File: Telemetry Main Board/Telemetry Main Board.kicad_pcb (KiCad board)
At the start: 2 copper layers, 107 x 144.2 mm, 26 parts, among them J1 8 pin ATM connector, J3 12 pin ATM connector, J4 SD to SPI (Molex nanofit), U1 LM7805_TO220, U2 LM7809_TO220, U3 NUCLEO-F446RE, U4 ISO1050DUB, U6 MCP6004, U8 ISO1050DUB

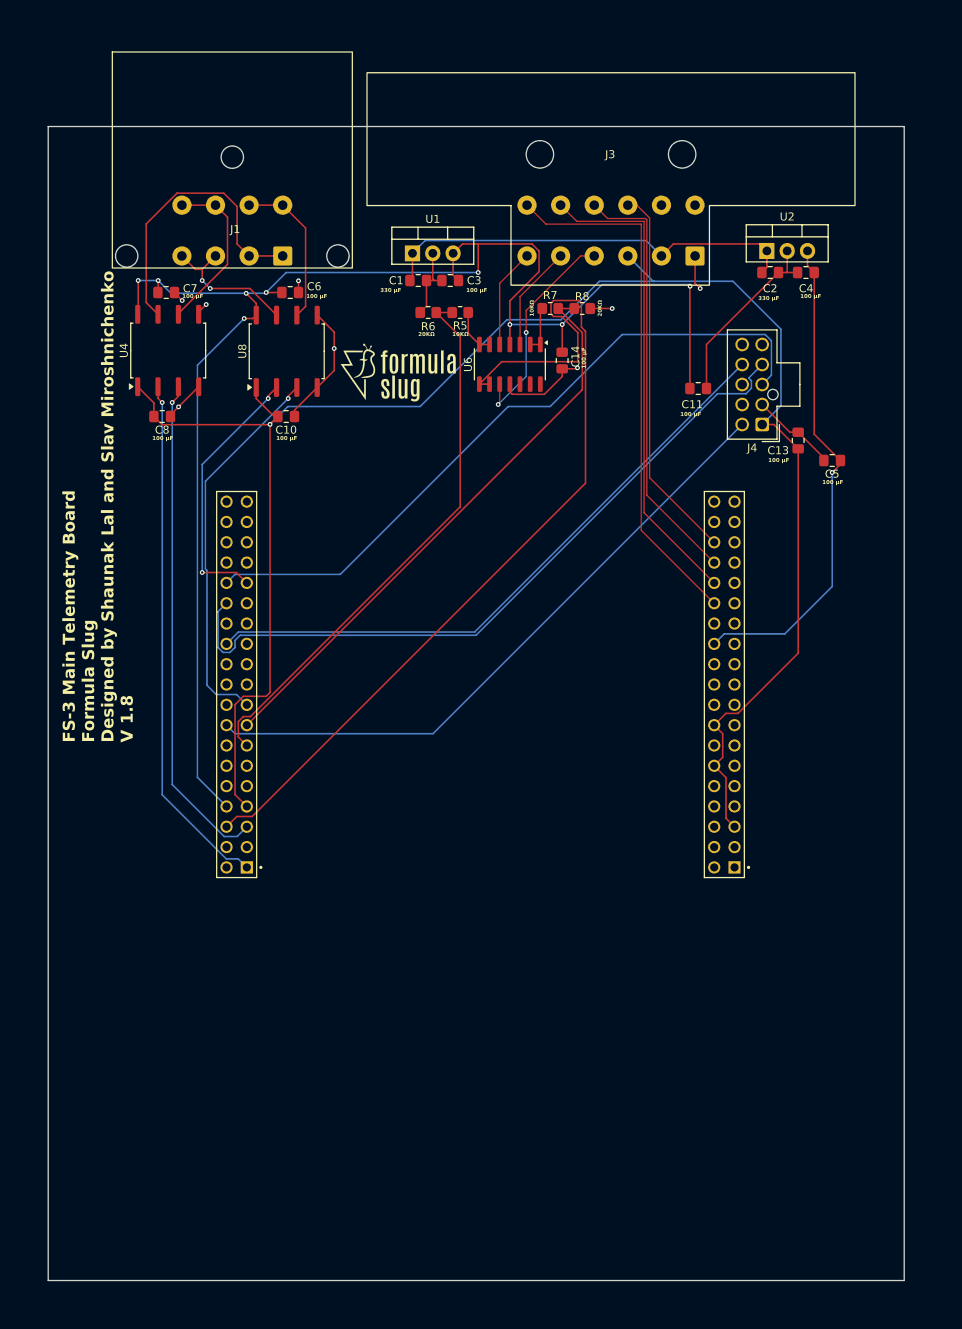
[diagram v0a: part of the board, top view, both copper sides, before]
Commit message: fixed telemetry main pcb
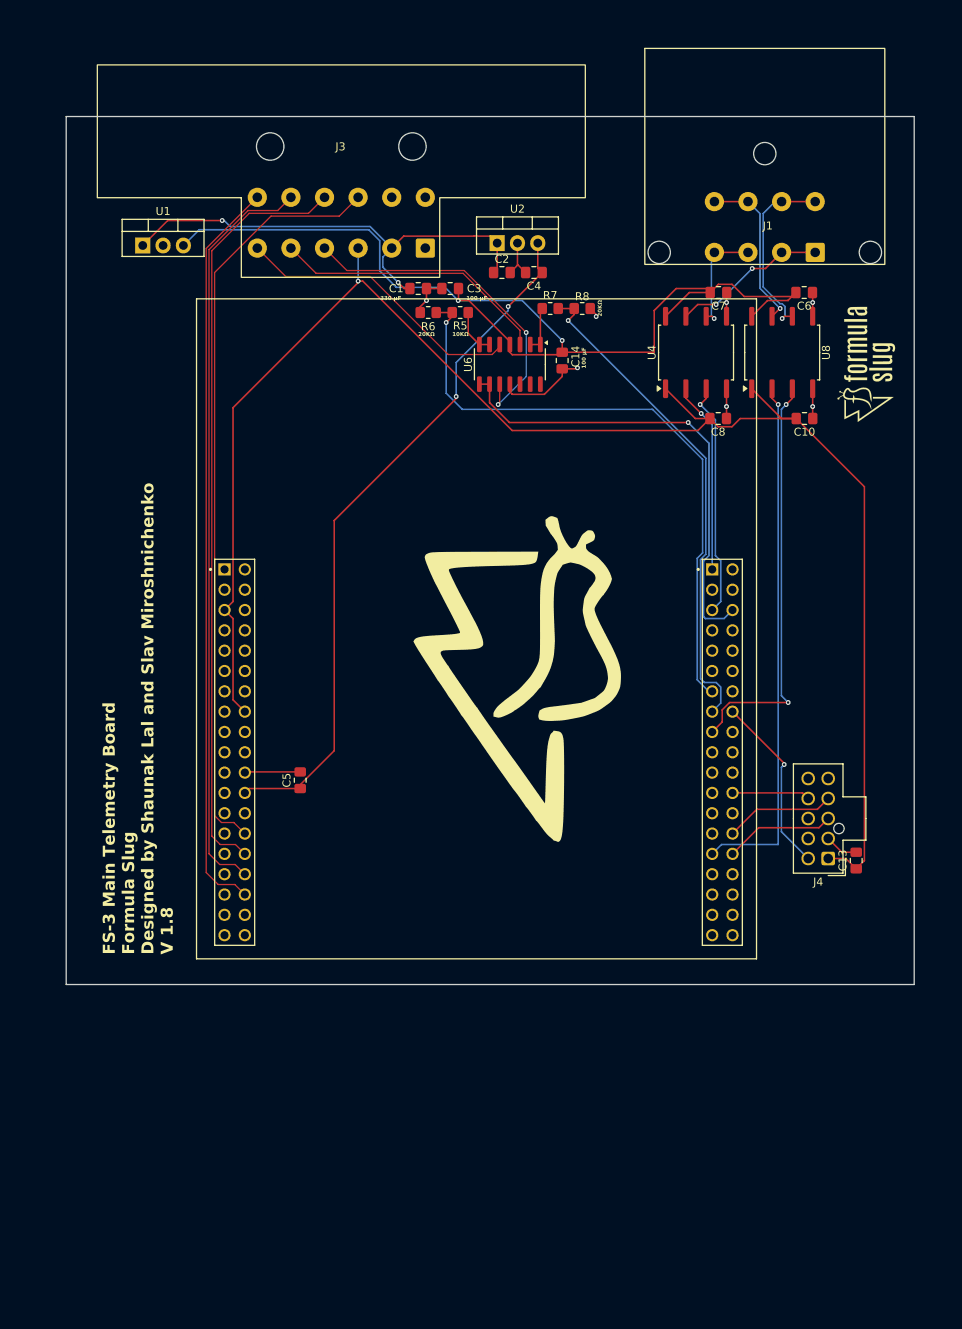
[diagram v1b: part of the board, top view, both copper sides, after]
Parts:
- removed C11: 100nf, Capacitor_SMD:C_0805_2012Metric_Pad1.18x1.45mm_HandSolder
- added G1: FS Logo, 1FS_2_Global_Footprint_Library:FS Logo Big, F.Cu at (132.0, 112.2)
- moved C5 77.6 mm to (105.2, 125.5), turned to 90 degrees
- moved C8 69.5 mm to (157.5, 80.2)
- moved C7 69.0 mm to (157.5, 64.5)
- moved J1 66.6 mm to (148.3, 61.0)
- moved U4 66.0 mm to (154.7, 72.0)
- moved C10 64.8 mm to (168.3, 80.2)
- moved C6 64.2 mm to (168.2, 64.5)
- moved U8 61.9 mm to (165.5, 72.0)
- moved G*** 58.5 mm to (176.0, 73.5), turned to 90 degrees
- moved J4 54.9 mm to (171.2, 135.2)
- moved C13 53.0 mm to (174.8, 135.5)
- moved C4 34.0 mm to (134.5, 62.0)
- moved J3 33.7 mm to (89.9, 42.6)
- moved U1 33.7 mm to (85.6, 58.6)
- moved U2 33.7 mm to (129.9, 58.3)
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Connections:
- J1 pad 3: CAN2_H -> CAN1_L
- J1 pad 4: CAN2_H -> CAN1_L
- J1 pad 5: CAN1_L -> CAN2_H
- J1 pad 6: CAN1_L -> CAN2_H
- U3 pad CN10_7: +3V3 -> unconnected-(U3B-AVDD-PadCN10_7)
- U3 pad CN10_8: +5V -> unconnected-(U3B-U5V-PadCN10_8)
- U3 pad CN7_12: +3V3 -> unconnected-(U3A-CN7_IOREF-PadCN7_12)
- U3 pad CN7_28: Acc Intake Temp -> Acc Intake Flow Rate
- U3 pad CN7_30: Acc Exhaust Temp -> Acc Intake Pressure
- U3 pad CN7_32: Acc Intake Pressure -> Acc Exhaust Temp
- U3 pad CN7_34: Acc Intake Flow Rate -> Acc Intake Temp
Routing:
- net SPI2_MISO: track 90.9 -> 13.8 mm
- net SPI2_SCK: track 87.2 -> 13.8 mm
- net SD Card Detect T/F: track 78.9 -> 9.75 mm
- net +5V: track 194.3 -> 126.4 mm, vias 9 -> 2
- net SPI2_CS: track 80.9 -> 22.7 mm, vias 0 -> 1
- net Steering Sensor 3V3: track 113.5 -> 59.2 mm, vias 0 -> 1
- net Acc Intake Flow Rate: track 47.3 -> 94.4 mm
- net CAN1_RX: track 65.6 -> 23.9 mm
- net Acc Intake Pressure: track 53.7 -> 95.1 mm
- net GND: track 87.7 -> 48.5 mm, vias 8 -> 7
- net Acc Exhaust Temp: track 60.1 -> 94.0 mm
- net CAN1_TX: track 62.6 -> 29.5 mm
- net CAN2_RX: track 33.1 -> 66.0 mm, vias 2 -> 1
- net Acc Intake Temp: track 66.4 -> 93.0 mm
- net +9V: track 61.8 -> 88.1 mm, vias 1 -> 2
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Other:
- board size 107 x 144.2 mm -> 106 x 108.5 mm
